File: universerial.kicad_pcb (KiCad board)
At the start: 2 copper layers, 19 parts, among them J1 USB_A, J2 Conn_01x06, U1 CH340G, Y1 12MHz

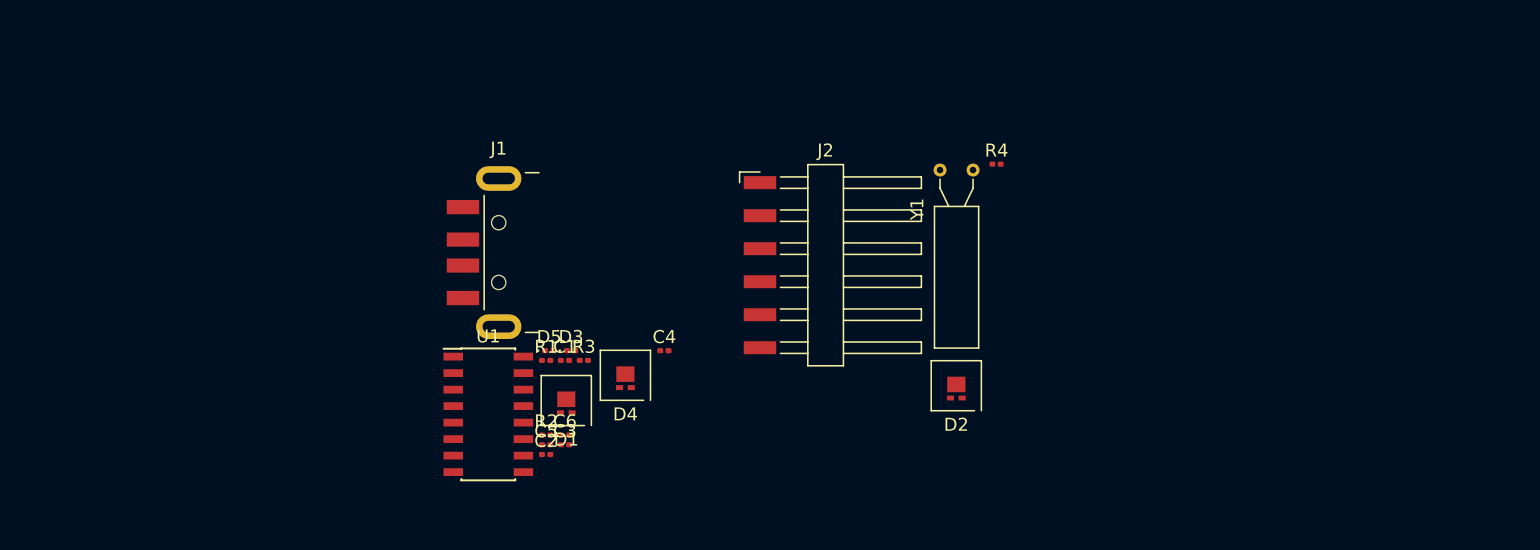
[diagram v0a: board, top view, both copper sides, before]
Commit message: Organize PCB.
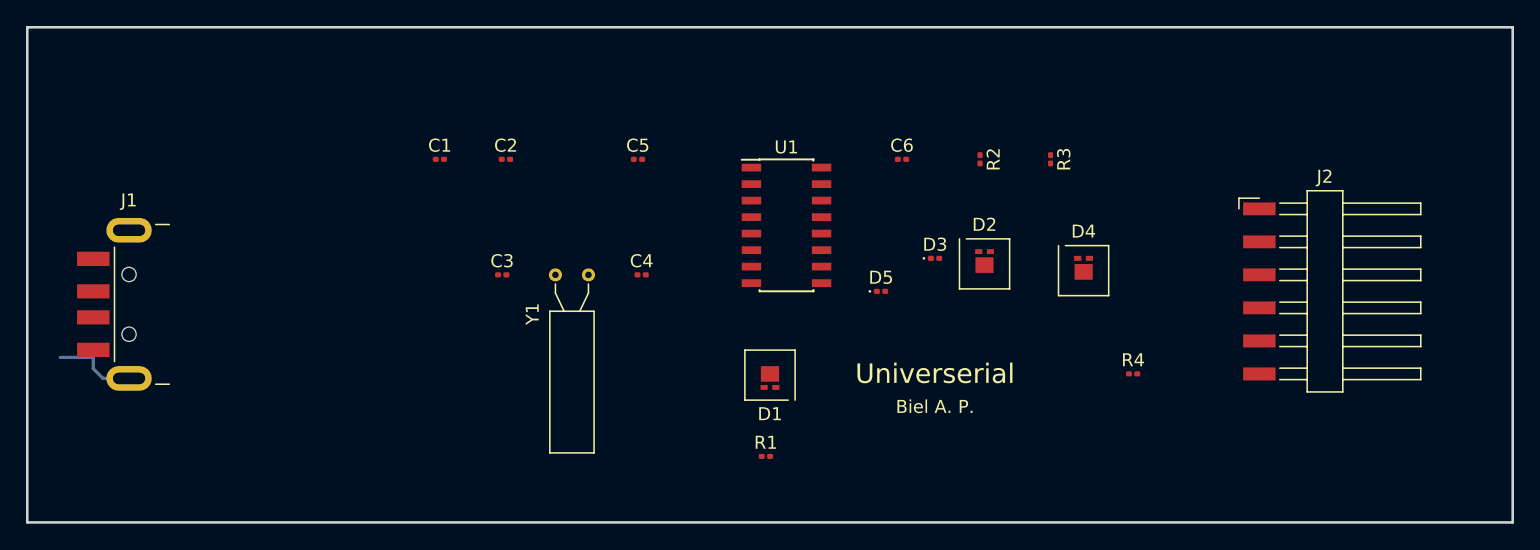
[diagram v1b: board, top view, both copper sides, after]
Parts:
- moved R2 39.6 mm to (174.9, 86.4), turned to 270 degrees
- moved R3 39.1 mm to (180.3, 86.4), turned to 270 degrees
- moved J2 38.5 mm to (201.9, 96.5)
- moved D4 36.4 mm to (182.9, 94.5), turned to 180 degrees
- moved C6 33.5 mm to (168.9, 86.4)
- moved Y1 30.7 mm to (142.2, 95.2)
- moved D3 28.9 mm to (171.4, 94.0)
- moved J1 28.7 mm to (116.3, 97.5)
- moved U1 27.2 mm to (160.0, 91.4)
- moved D5 25.9 mm to (167.3, 96.5)
- moved C5 23.1 mm to (148.6, 86.4)
- moved C2 22.9 mm to (138.4, 86.4)
- moved R4 19.3 mm to (186.7, 102.9)
- moved R1 18.4 mm to (158.4, 109.2)
- moved C1 18.2 mm to (133.3, 86.4)
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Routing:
- net GND: track 0.00 -> 6.47 mm
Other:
- board outline added: 114.3 x 38.1 mm
- board text added: "Biel A. P."
- board text added: "Universerial"
